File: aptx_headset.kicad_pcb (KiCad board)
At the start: 2 copper layers, 65.4 x 32.3 mm, 61 parts, among them J1 AudioJack4, J2 Conn_01x03, SW1 vol+, SW2 vol-, SW3 next, SW4 prev, SW5 pp/call, SW6 mute, U1 OPA1664, U2 CSR8645, U3 OPA1664, U4 LM358

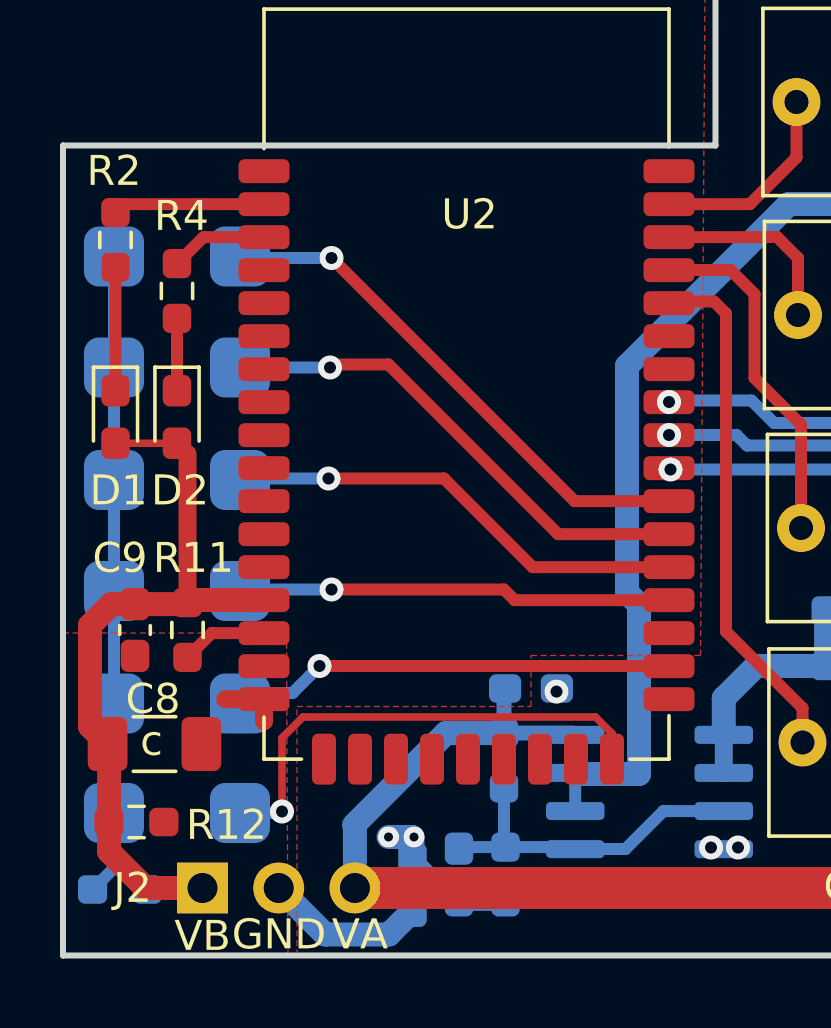
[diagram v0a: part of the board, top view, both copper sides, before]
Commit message: move buttons
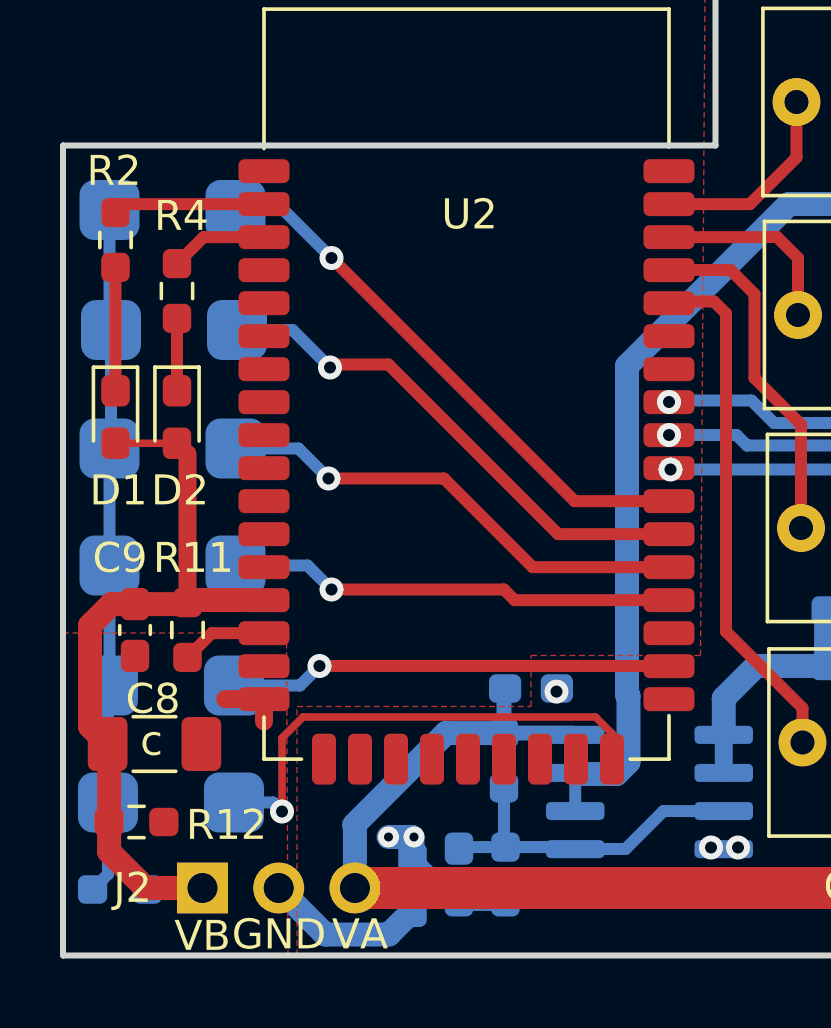
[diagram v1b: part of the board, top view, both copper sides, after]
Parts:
- moved SW1 1.56 mm to (89.5, 76.3)
- moved SW2 1.25 mm to (89.5, 80.3)
- moved SW3 1.06 mm to (89.5, 84.2)
- moved SW4 0.86 mm to (89.5, 88.2)
- moved SW5 0.63 mm to (89.5, 92.2)
- moved SW6 0.40 mm to (89.5, 96.0)
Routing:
- net Net-(R21-Pad2): track 21.4 -> 22.9 mm
- net /VOL+: track 17.7 -> 18.5 mm
- net /VGND_L: track 28.3 -> 27.6 mm
- net /VOL-: track 16.7 -> 17.3 mm
- net /NEXT: track 15.5 -> 16.1 mm
